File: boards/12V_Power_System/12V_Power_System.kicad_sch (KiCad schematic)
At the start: 21 parts, among them J1 Screw_Terminal_01x02, J10 Motor_Controller_5_Term_01x02, J2 Motor_Controller_1_Term_01x02, J4 Motor_Controller_2_Term_01x02, J6 Motor_Controller_1_Term_01x02, J8 Motor_Controller_4_Term_01x02, U1 irhapsody_relay_12vdc_8060a_1, U2 irhapsody_relay_12vdc_8060a_2, U3 irhapsody_relay_12vdc_8060a_3, U4 irhapsody_relay_12vdc_8060a_4, U5 irhapsody_relay_12vdc_8060a_5

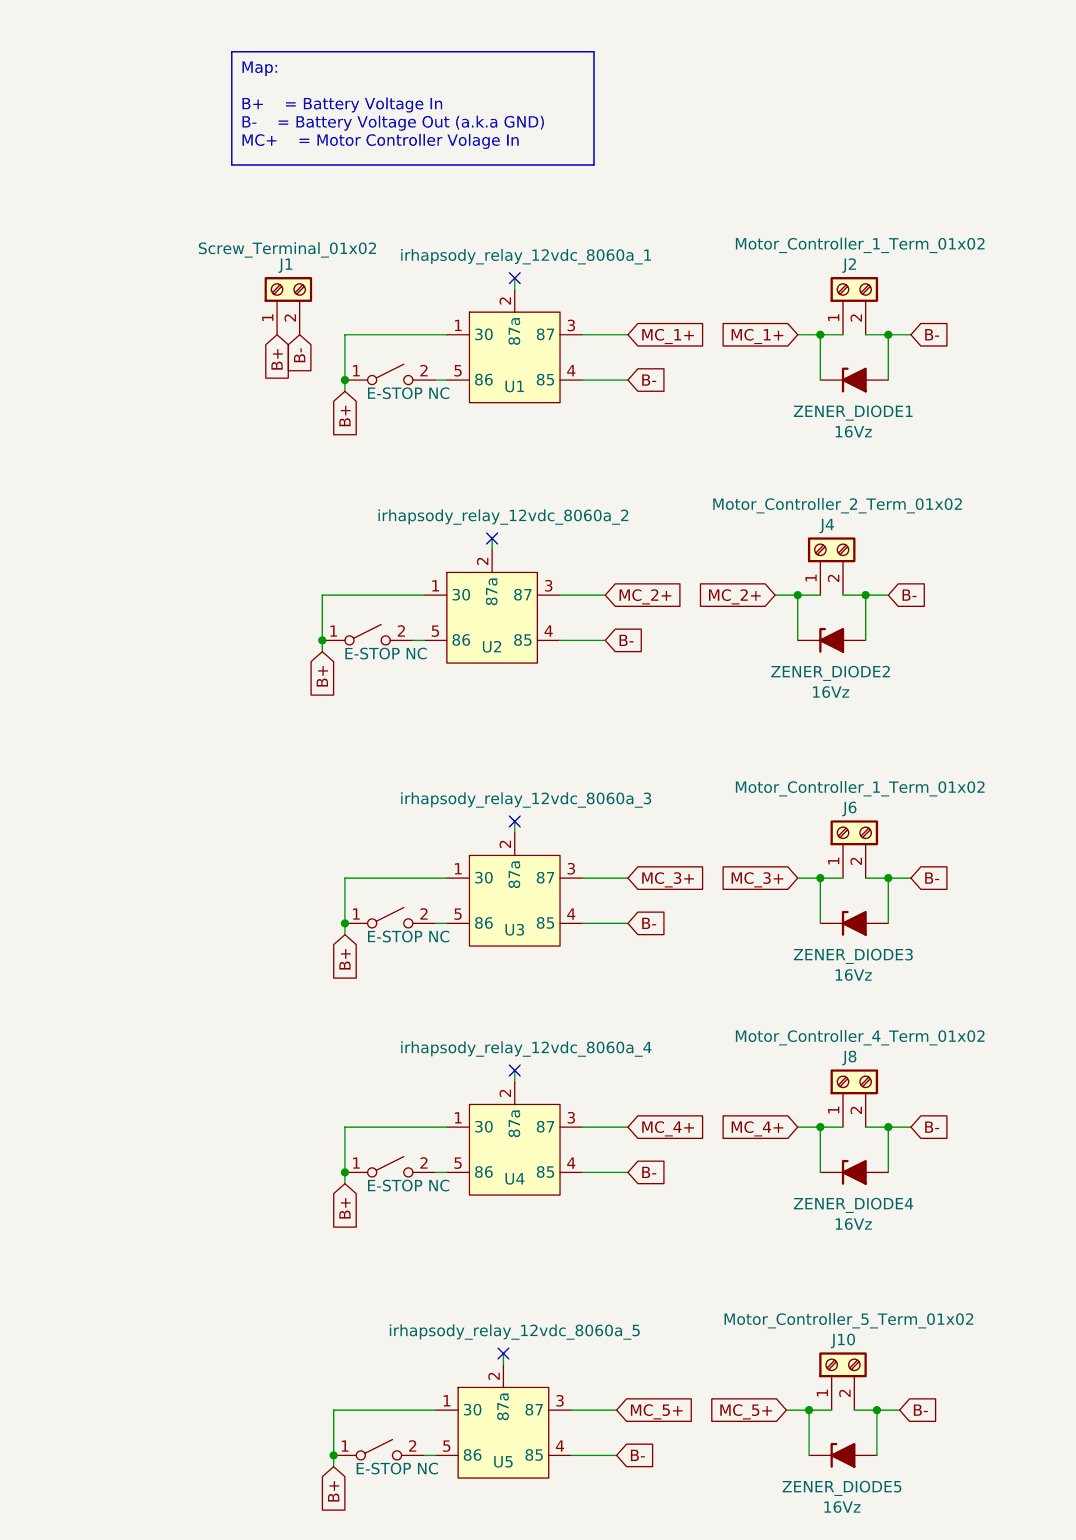
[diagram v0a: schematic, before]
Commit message: updated schematic
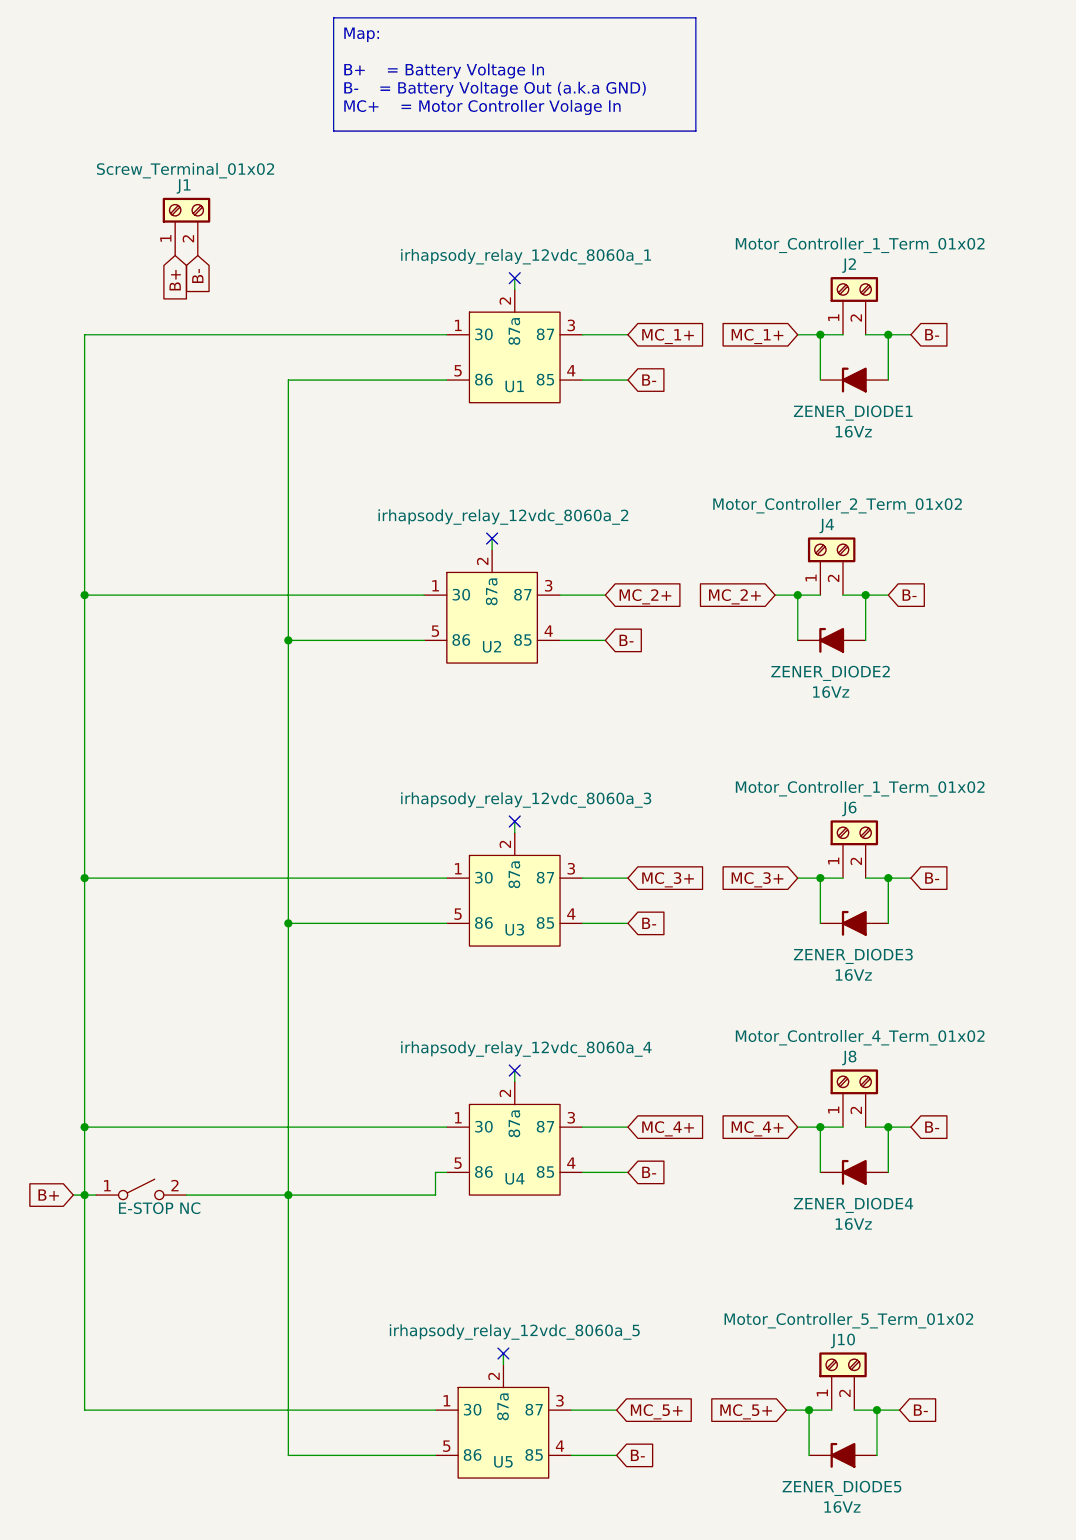
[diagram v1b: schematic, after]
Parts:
- removed E-STOP1, E-STOP2, E-STOP3, E-STOP4: E-STOP NC, symbol Switch:SW_DPST_x2
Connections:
- net at U3.5 (86): now also E-STOP5.2 (B), U1.5 (86), U2.5 (86), U4.5 (86), U5.5 (86)
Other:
- moved on the sheet: J1
